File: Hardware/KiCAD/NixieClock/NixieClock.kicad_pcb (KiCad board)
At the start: 2 copper layers, 7 parts

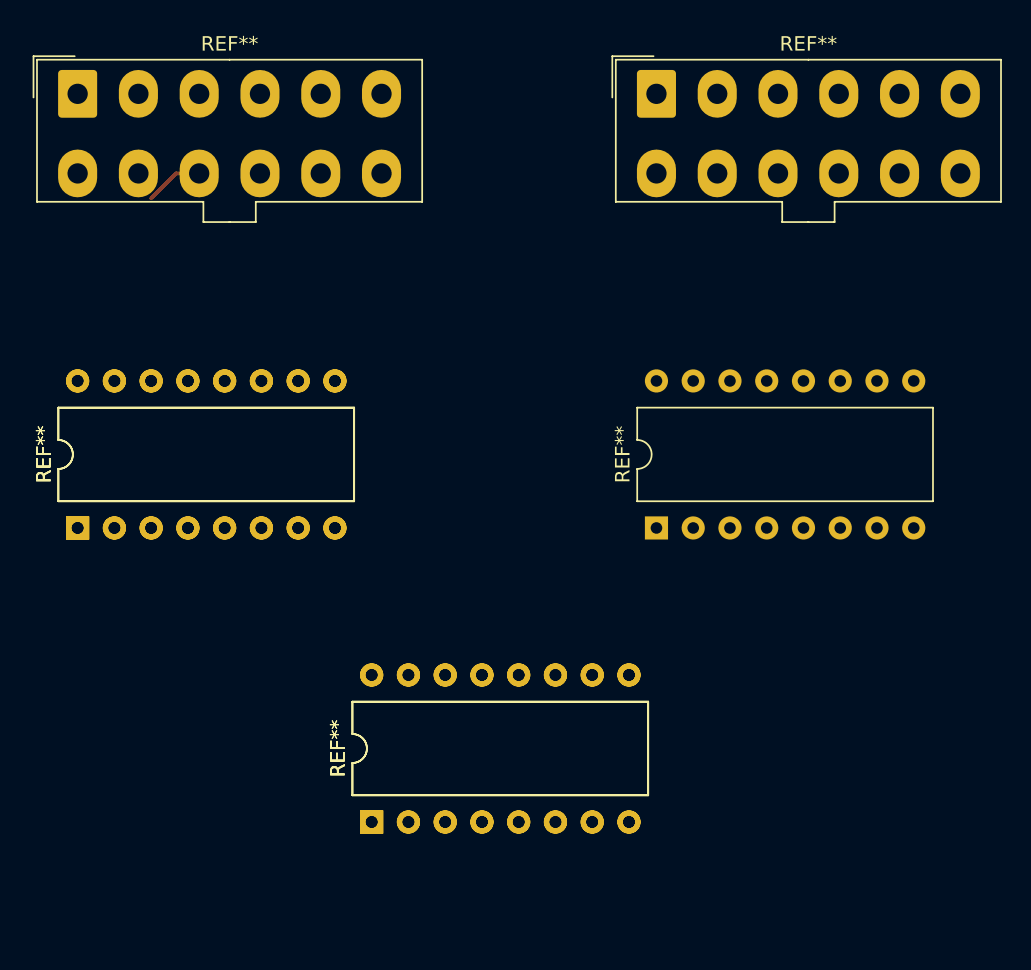
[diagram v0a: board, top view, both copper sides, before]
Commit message: KiCAD Progress
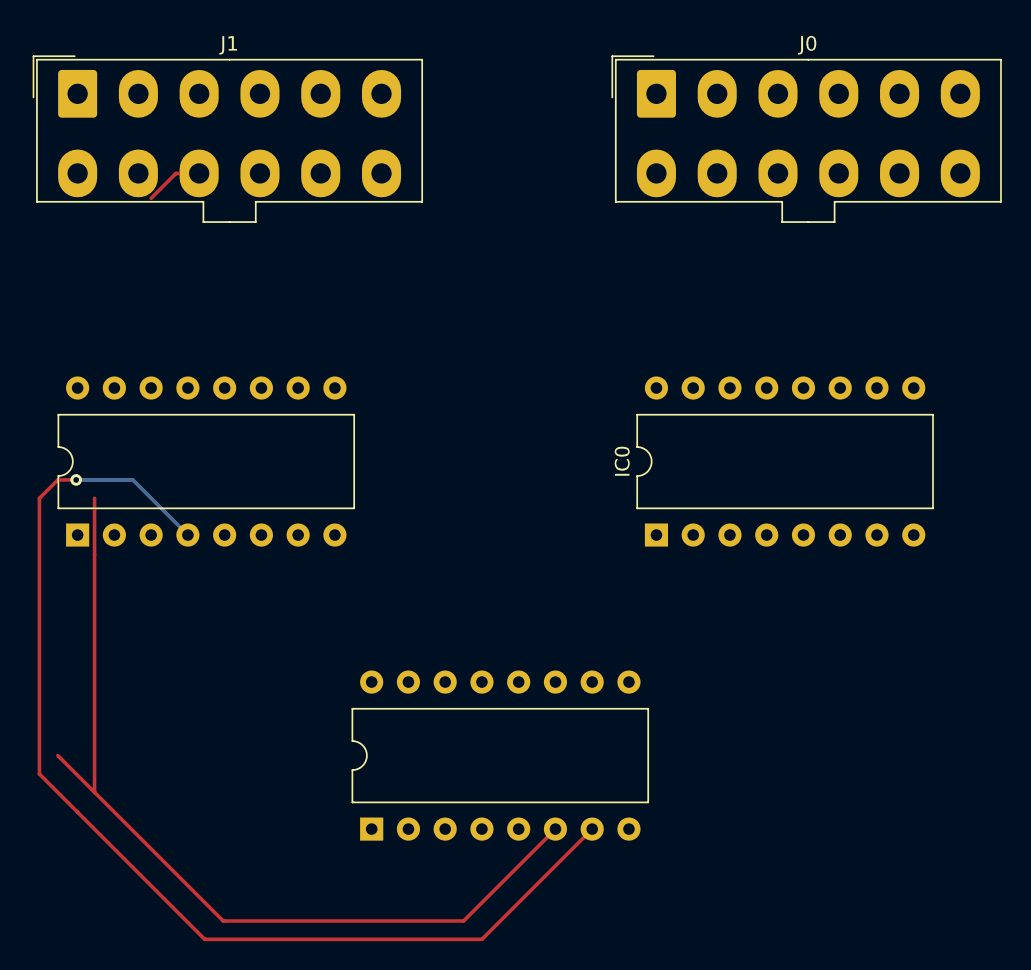
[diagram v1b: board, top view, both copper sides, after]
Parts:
- removed REF** (x2): DIP-16_W10.16mm, Package_DIP:DIP-16_W10.16mm
- J0, J1: renamed from REF**; value Molex_Mini-Fit_Jr_5566-12A_2x06_P4.20mm_Vertical -> (none)
- moved IC0 0.49 mm to (55.3, 58.4)
- moved IC2 0.49 mm to (15.3, 58.4)
- moved IC1 0.49 mm to (35.7, 78.7)
- renumbered REF** to IC0, REF** to IC1, REF** to IC2
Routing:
- net (no net): track 4.03 -> 143.6 mm, vias 0 -> 1
